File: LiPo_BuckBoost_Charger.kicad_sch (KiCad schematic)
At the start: 53 parts, among them J2 Type-C_6P, J3 Conn_01x01, J4 Conn_01x01, J7 JST PH Connector, U1 TP4056, U2 DW01A, U3 FS8205A, U4 TPS63020

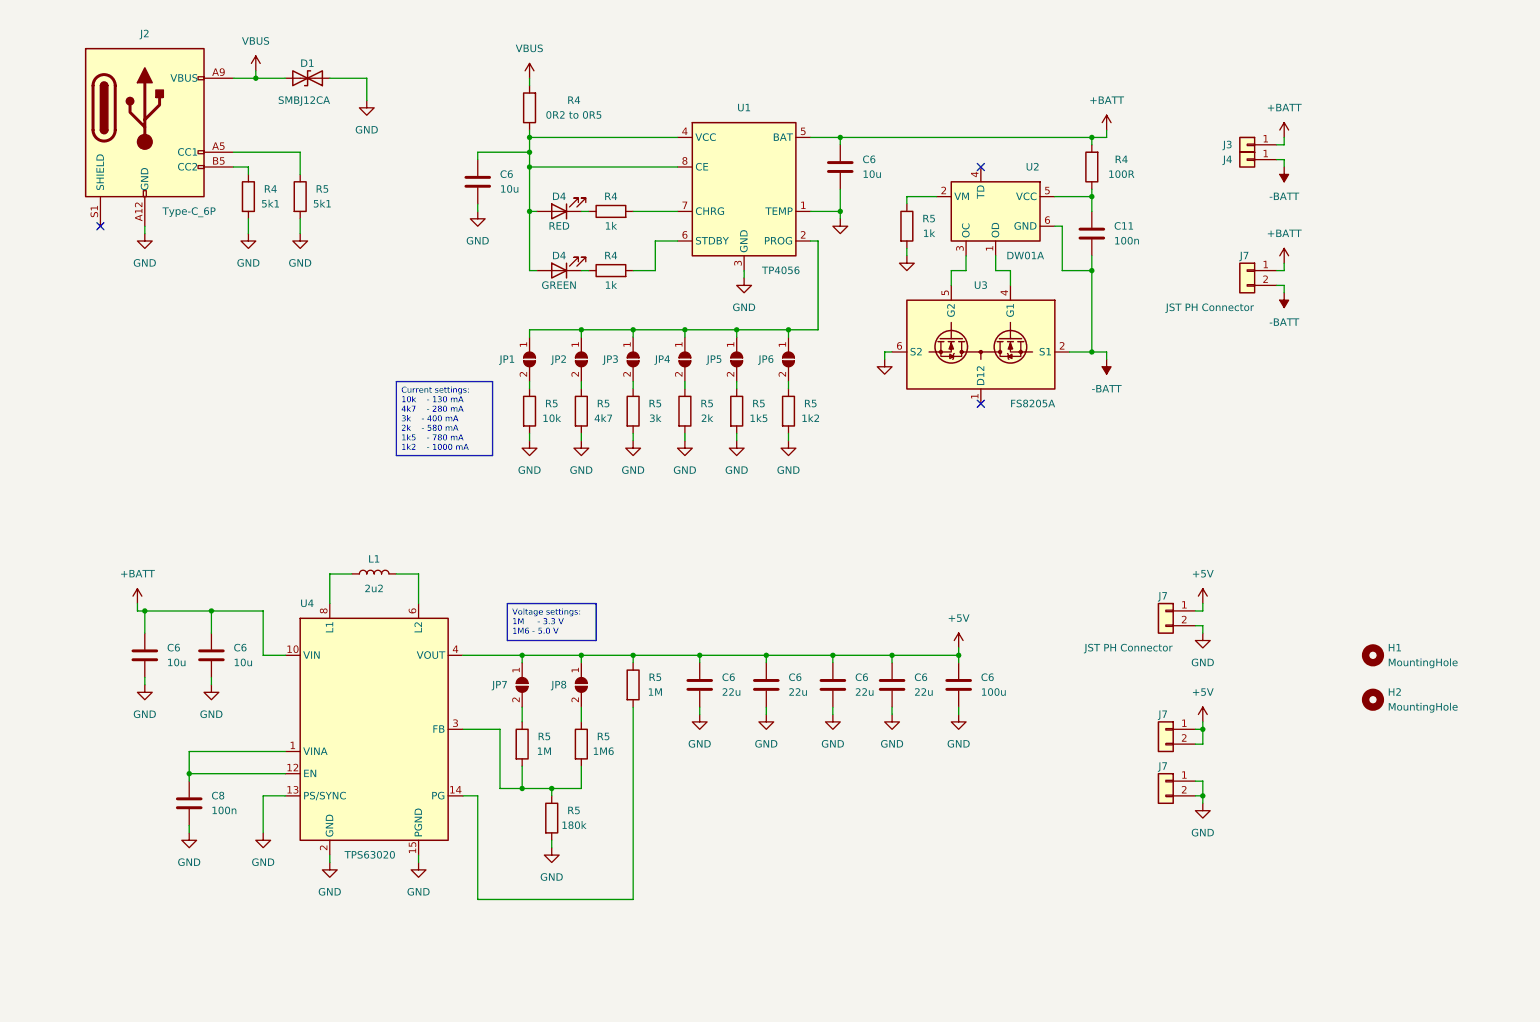
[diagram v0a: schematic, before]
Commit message: schematic update, added imgs
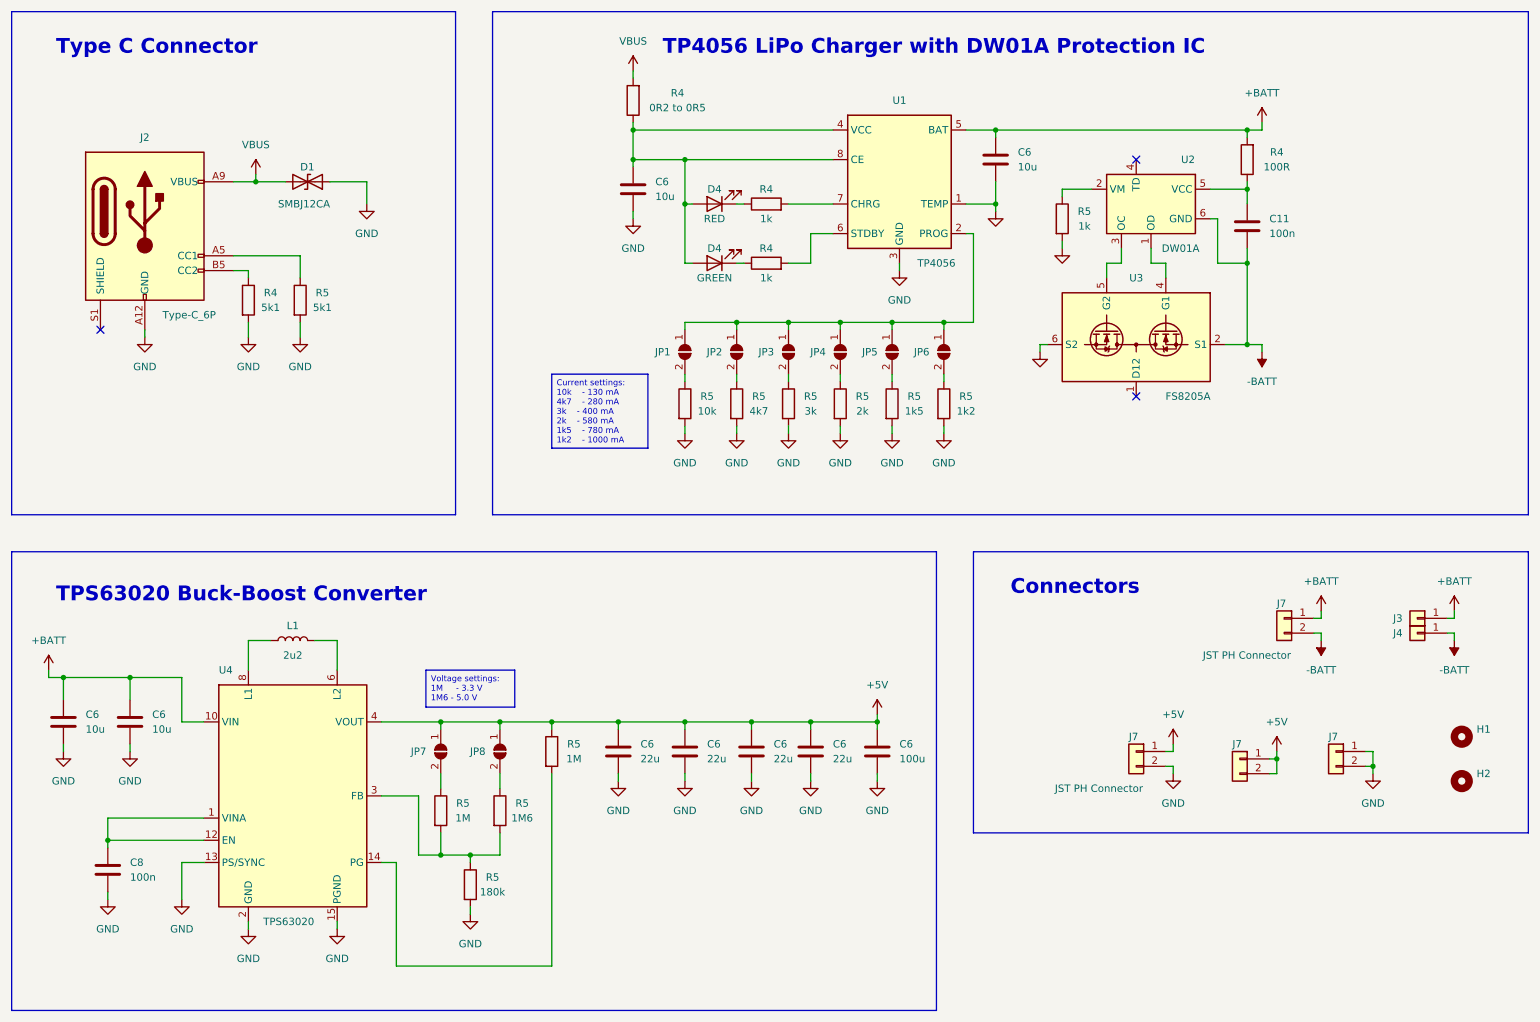
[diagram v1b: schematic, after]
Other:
- note added: "Connectors"
- note added: "TP4056 LiPo Charger with DW01A Protection IC"
- note added: "TPS63020 Buck-Boost Converter"
- note added: "Type C Connector"
- company: (none) -> Potpurri
- title: (none) -> LiPo Buck-Boost Charger
- moved on the sheet: C11, C6, C8, D1, D4, H1, H2, J2, J3, J4, J7, JP1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
